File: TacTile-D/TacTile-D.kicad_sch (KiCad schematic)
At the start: 13 parts, among them J18 Conn_01x04, J18 Conn_01x06, J19 Conn_01x05, J19 Conn_01x06, J20 Conn_01x02, J20 Conn_01x06, J21 Conn_01x02, J21 Conn_01x06, U11 74LS04, U12 74HC595, U13 74HC590, U2 4011, U6 74HC08

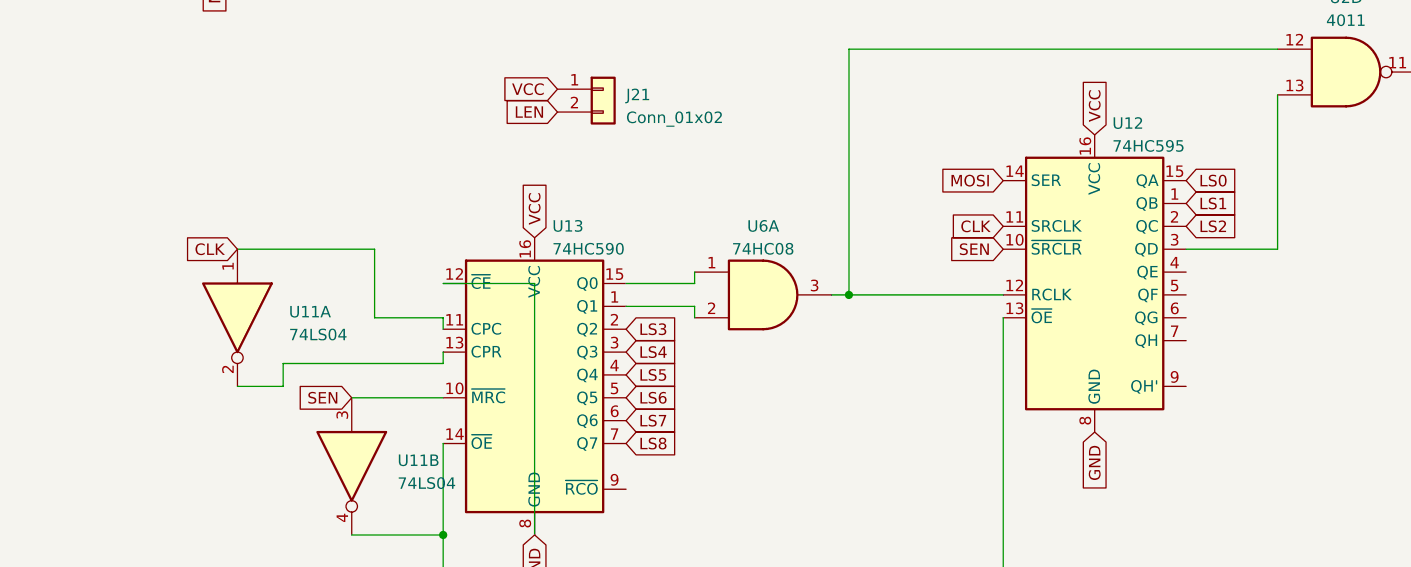
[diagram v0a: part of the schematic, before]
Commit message: Fixed issues with D board and rerouted
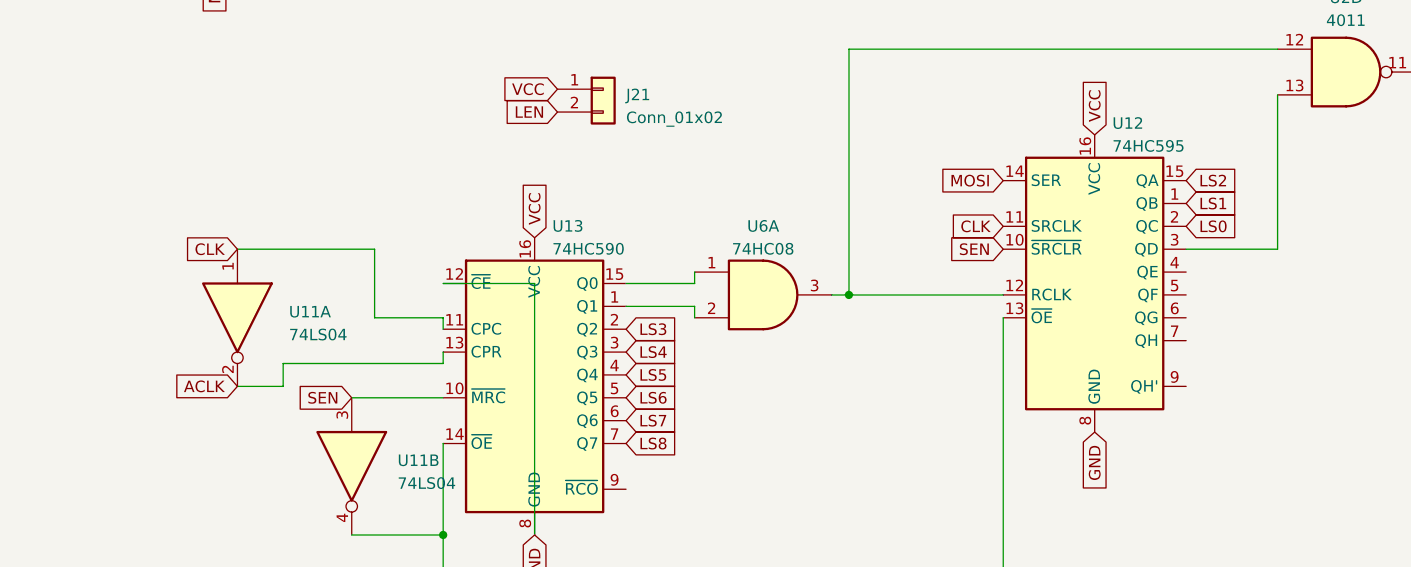
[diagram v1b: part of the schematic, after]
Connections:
- net LS0: now also U12.2 (QC); no longer U12.15 (QA)
- net LS2: now also U12.15 (QA); no longer U12.2 (QC)
- net ACLK: now reaches U11.2, U13.13 (CPR)
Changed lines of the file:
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@@
     )
   )
-  (global_label "LS2" (shape input) (at 149.86 81.28 0) (fields_autoplaced)
+  (global_label "LS2" (shape input) (at 149.86 76.2 0) (fields_autoplaced)
     (effects (font (size 1.27 1.27)) (justify left))
-    (property "Intersheetrefs" "${INTERSHEET_REFS}" (at 156.2129 81.28 0)
+    (property "Intersheetrefs" "${INTERSHEET_REFS}" (at 156.2129 76.2 0)
       (effects (font (size 1.27 1.27)) (justify left) hide)
     )
@@
     )
   )
+  (global_label "ACLK" (shape input) (at 44.45 99.06 180) (fields_autoplaced)
+    (effects (font (size 1.27 1.27)) (justify right))
+    (property "Intersheetrefs" "${INTERSHEET_REFS}" (at 36.8875 99.06 0)
+      (effects (font (size 1.27 1.27)) (justify right) hide)
+    )
+  )
   (global_label "LS3" (shape input) (at 80.01 24.13 180) (fields_autoplaced)
     (effects (font (size 1.27 1.27)) (justify right))
@@
     )
   )
-  (global_label "LS0" (shape input) (at 149.86 76.2 0) (fields_autoplaced)
+  (global_label "LS0" (shape input) (at 149.86 81.28 0) (fields_autoplaced)
     (effects (font (size 1.27 1.27)) (justify left))
-    (property "Intersheetrefs" "${INTERSHEET_REFS}" (at 156.2129 76.2 0)
+    (property "Intersheetrefs" "${INTERSHEET_REFS}" (at 156.2129 81.28 0)
       (effects (font (size 1.27 1.27)) (justify left) hide)
     )
